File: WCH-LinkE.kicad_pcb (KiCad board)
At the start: 2 copper layers, 38.1 x 17.8 mm, 35 parts, among them J2 Conn_02x05_Odd_Even, J3 USB_C_Receptacle_USB3.1_16P, SW1 SW_Push, SW2 SW_Push, U1 RT9080-33GJ5, U2 CH32V305FBP6, U3 CH217K, U4 CH217K, Y2 12M

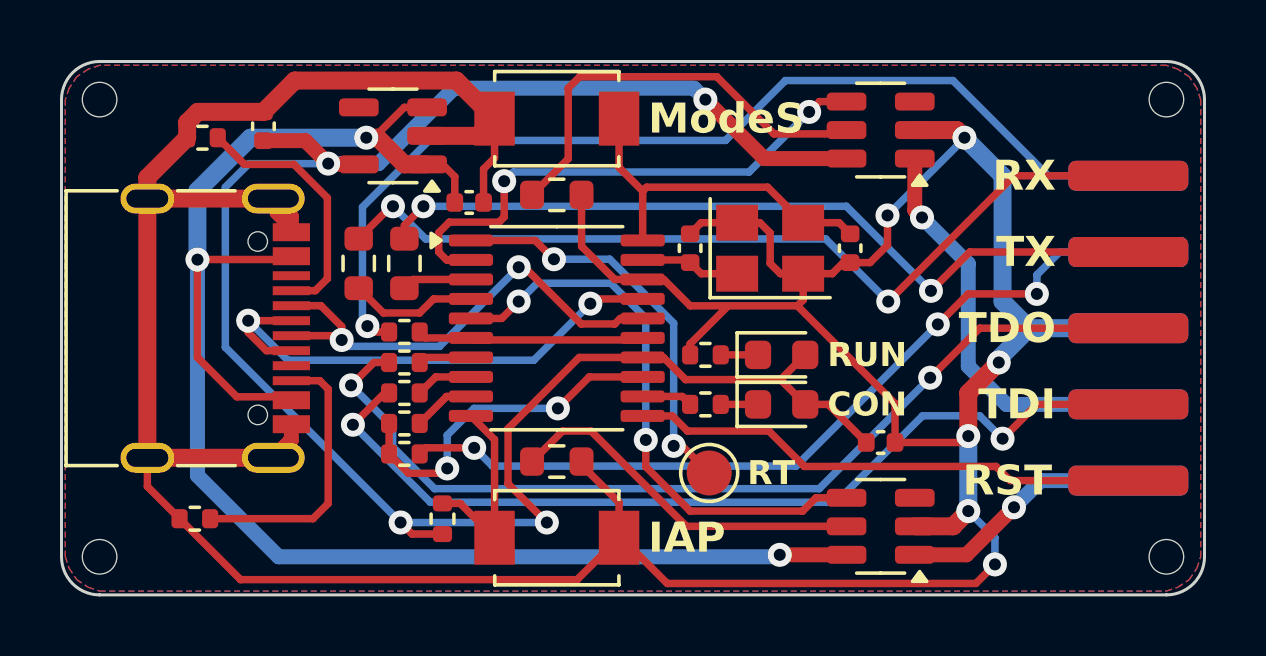
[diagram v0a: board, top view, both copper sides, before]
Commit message: v1.1.0 pre-release
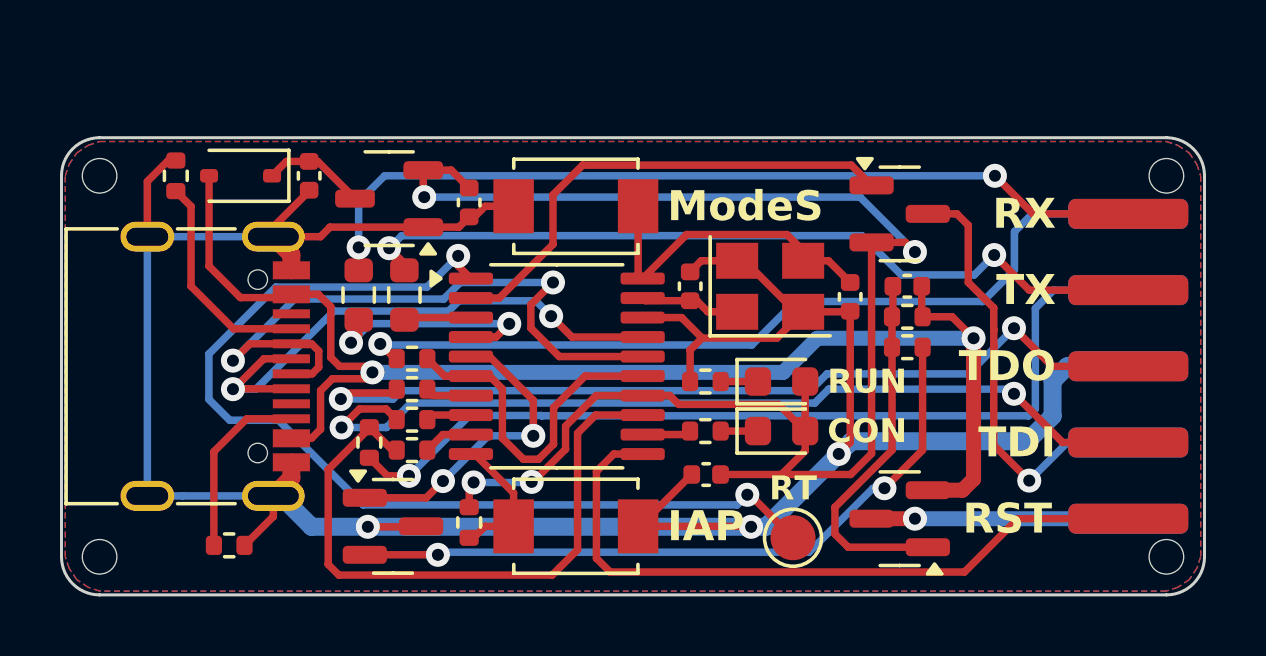
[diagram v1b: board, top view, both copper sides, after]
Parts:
- removed U1: RT9080-33GJ5, Package_TO_SOT_SMD:TSOT-23-5
- removed U3, U4: CH217K, Package_TO_SOT_SMD:SOT-23-6
- added C6: 0.1u, Capacitor_SMD:C_0402_1005Metric, F.Cu at (155.2, 116.7)
- added D3: 1N5819WS, Diode_SMD:D_SOD-323, F.Cu at (133.0, 113.0)
- added Q1: AO3401A, Package_TO_SOT_SMD:SOT-23, F.Cu at (154.9, 114.3)
- added Q2: AO3401A, Package_TO_SOT_SMD:SOT-23, F.Cu at (154.9, 124.5)
- added Q3: AO3401A, Package_TO_SOT_SMD:SOT-23, F.Cu at (138.0, 124.7)
- added U5: XC6206P332MR-G, Package_TO_SOT_SMD:SOT-23-3, F.Cu at (137.9, 113.8)
- C4: value 10u -> 1u
- C5: value 100n -> 0.1u
- J3: value USB_C_Receptacle_USB3.1_16P -> TYPE-C16PIN
- R13: value 150k -> 47k; footprint Resistor_SMD:R_0603_1608Metric -> Resistor_SMD:R_0402_1005Metric
- R14: value 300k -> 100k; footprint Resistor_SMD:R_0603_1608Metric -> Resistor_SMD:R_0402_1005Metric
- R8, R9: value 1k -> 5.1k
- moved R14 12.7 mm to (155.2, 118.7)
- moved R13 12.6 mm to (155.2, 117.7), turned to 180 degrees
- moved C4 7.31 mm to (140.6, 113.9), turned to -90 degrees
- moved C5 5.91 mm to (148.5, 123.0), turned to 180 degrees
- moved C2 5.41 mm to (135.3, 113.0), turned to -90 degrees
- moved TP1 3.53 mm to (151.4, 125.1)
- moved SW1 2.99 mm to (144.1, 114.0)
- moved H2 2.54 mm to (128.3, 113.0)
- moved H3 2.54 mm to (163.8, 113.0)
- moved C1 1.62 mm to (153.3, 117.1)
- moved R11 1.55 mm to (130.8, 113.0), turned to -90 degrees
- moved R12 1.45 mm to (132.6, 125.3), turned to 180 degrees
- moved C3 1.27 mm to (148.0, 116.7)
- moved J2 1.27 mm to (162.6, 119.4)
- moved J3 1.27 mm to (130.9, 119.4)
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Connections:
- C2 pad 1: +5V -> Net-(D3-K)
- R13 pad 1: Net-(U3-ISET) -> +5V
- R13 pad 2: GND -> Net-(Q2-G)
- R14 pad 1: Net-(U4-ISET) -> Net-(Q2-G)
- R14 pad 2: GND -> Net-(Q3-S)
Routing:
- net GND: track 133.5 -> 94.0 mm, vias 6 -> 3
- net Net-(Q3-S): track 0.00 -> 23.5 mm, vias 0 -> 2
- net Net-(U2-~{RST}): track 13.5 -> 33.8 mm
- net Net-(U4-ISET): track 14.7 -> 0.00 mm
- net +3V3: track 65.8 -> 51.3 mm
- net Net-(Q2-G): track 0.00 -> 12.3 mm
- net Net-(U3-ISET): track 12.2 -> 0.00 mm
- net +5V: track 55.6 -> 45.3 mm, vias 3 -> 2
- net /D_SWDIO: track 11.7 -> 21.5 mm, vias 2 -> 0
- net /PB12: track 19.2 -> 10.3 mm
- net /RST: track 17.1 -> 23.3 mm
- net /USB_N: track 16.3 -> 22.4 mm
- net /SWCLK/TCK: track 33.4 -> 28.3 mm
- net /D_SWCLK: track 7.57 -> 11.4 mm
- net Net-(U2-PB11): track 4.28 -> 7.78 mm, vias 0 -> 2
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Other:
- board size 38.1 x 17.8 mm -> 38.1 x 15.2 mm
